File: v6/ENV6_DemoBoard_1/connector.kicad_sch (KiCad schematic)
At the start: 9 parts, among them J501 Conn_02x16_Odd_Even, J502 Conn_02x04_Odd_Even, J503 Conn_02x16_Odd_Even, J504 Conn_02x04_Odd_Even, J505 Conn_02x16_Odd_Even

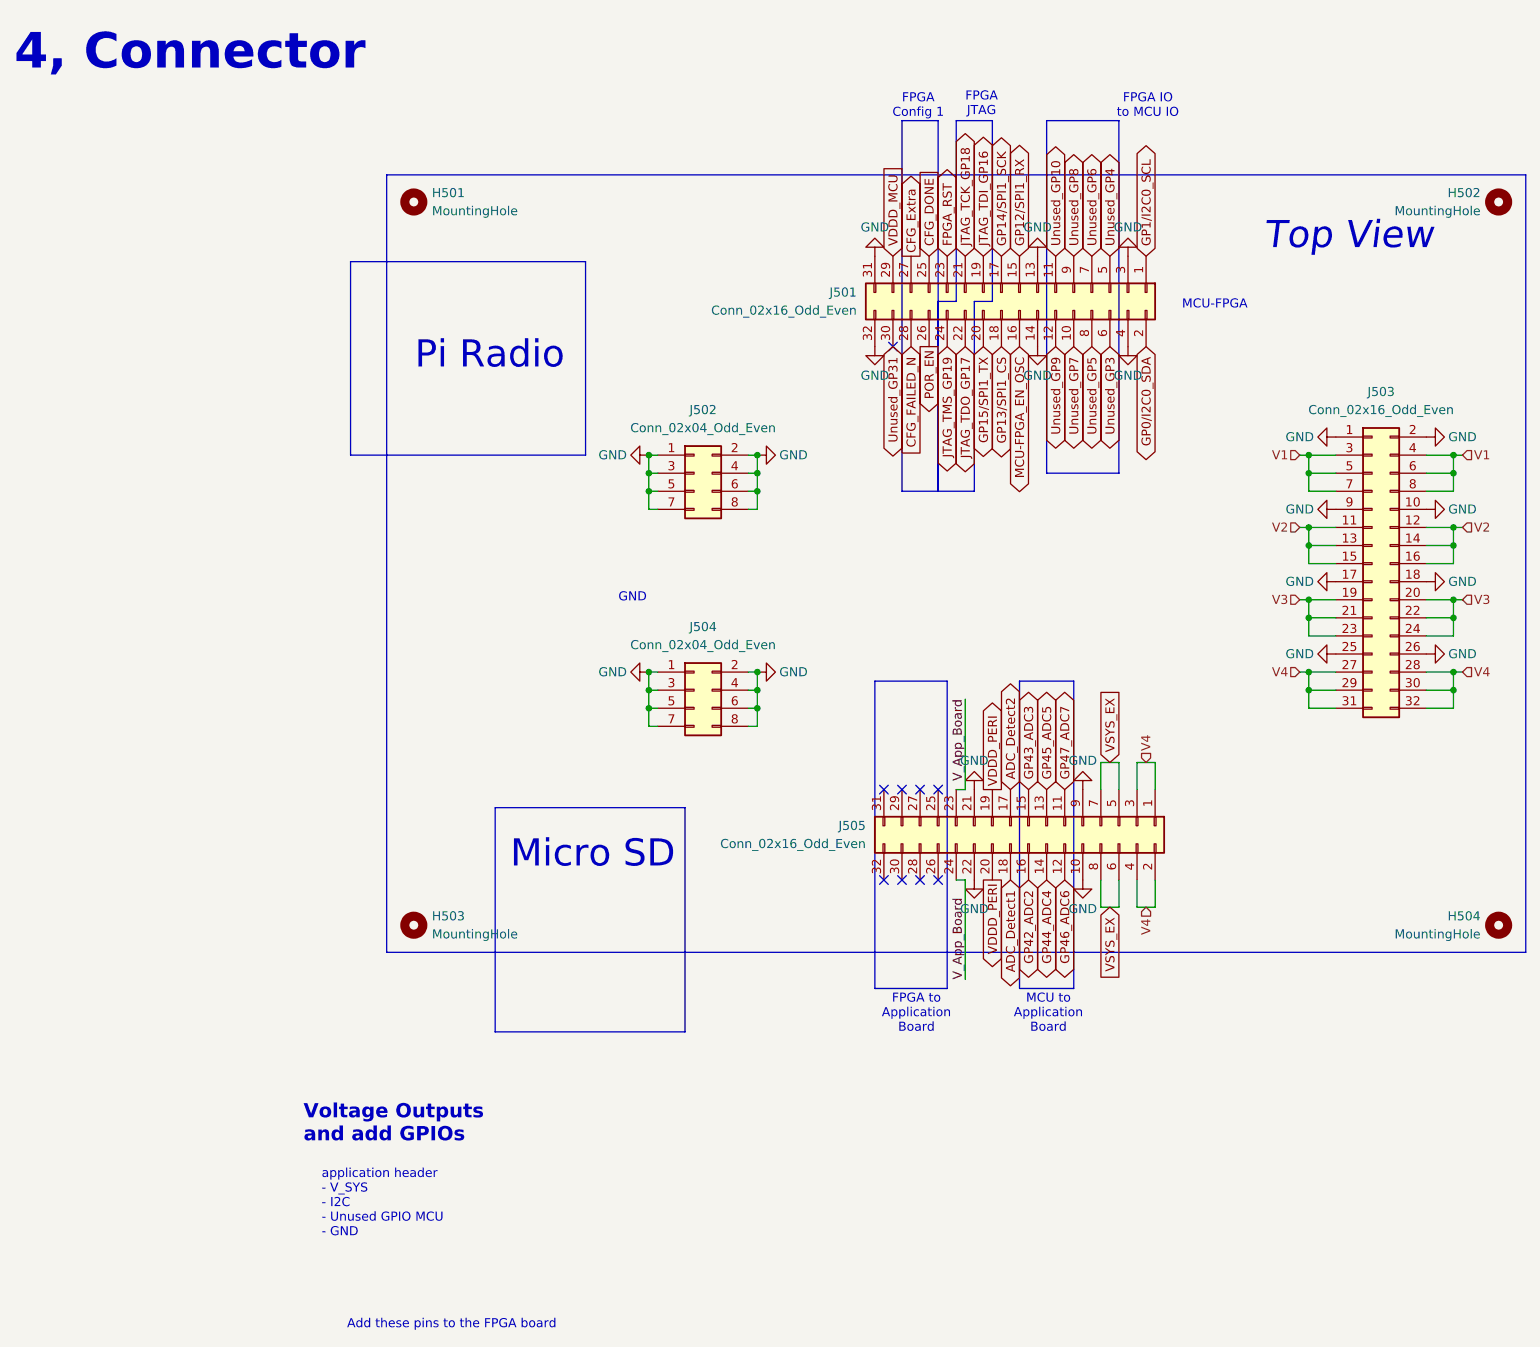
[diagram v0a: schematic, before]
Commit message: first rev Base Board pcb layout
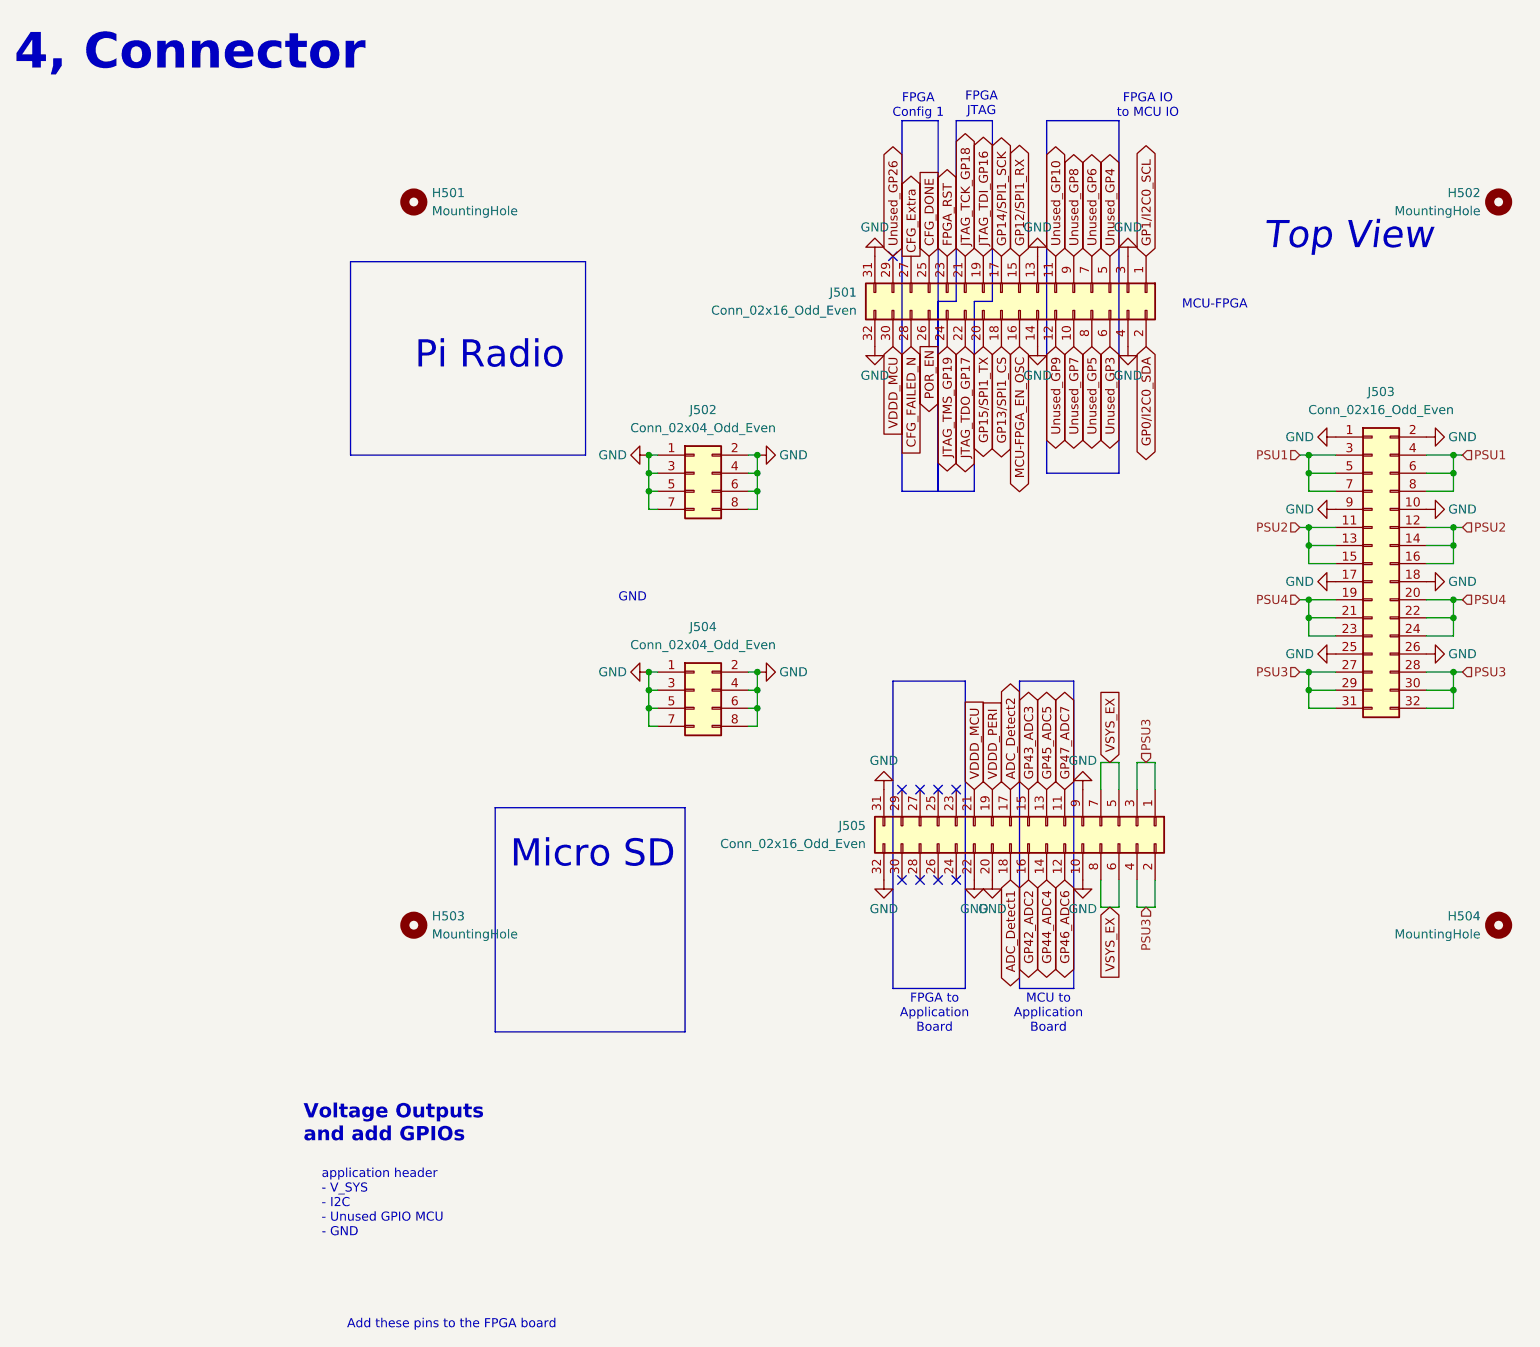
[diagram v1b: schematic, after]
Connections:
- net Unused_GP31 is gone; now on net VDDD_MCU: J501.30 (Pin_30)
- net GND: now also J505.20 (Pin_20), J505.31 (Pin_31), J505.32 (Pin_32); no longer J505.21 (Pin_21)
- net VDDD_MCU: now also J505.21 (Pin_21); no longer J501.29 (Pin_29)
- net VDDD_PERI: no longer J505.20 (Pin_20)
- net V1 renamed PSU1
- net V2 renamed PSU2
- net V3 renamed PSU4
- net V4 renamed PSU3
- net V_App_Board: no longer names the net of J505.23 (Pin_23)
- net V_App_Board: no longer J505.24 (Pin_24)
- new net Unused_GP26: J501.29 (Pin_29)
